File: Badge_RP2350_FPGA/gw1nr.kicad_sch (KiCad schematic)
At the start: 18 parts, among them U2 GW1N-LV9QN88C6_I5_, U6 W25Q32JVSS

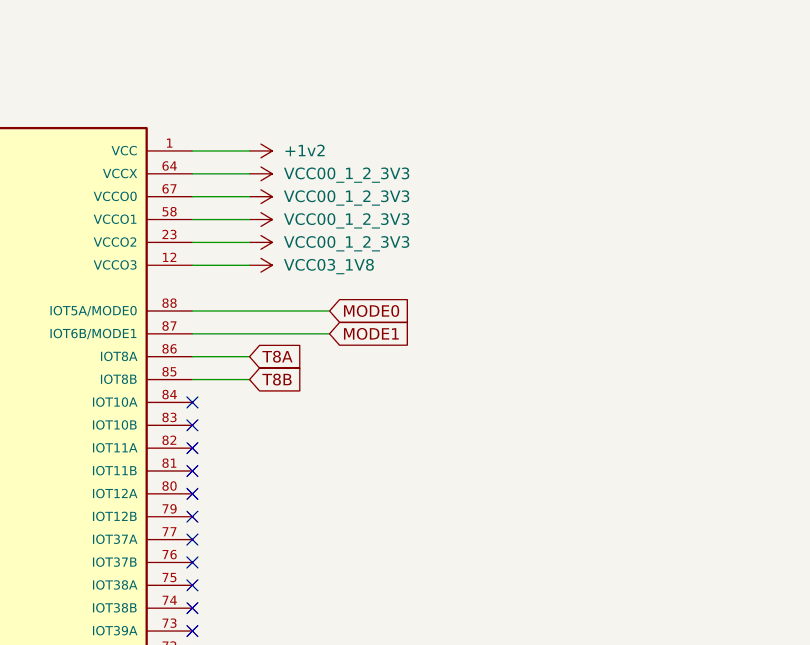
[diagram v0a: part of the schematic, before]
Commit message: put pull up to mode1, pull down to mode0
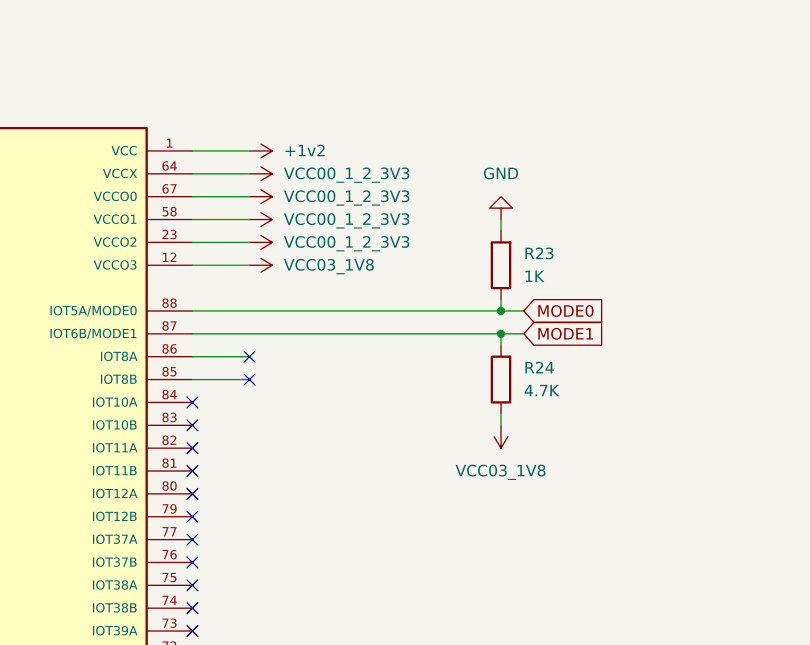
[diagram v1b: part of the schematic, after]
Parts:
- added R23: 1K, Resistor_SMD:R_0402_1005Metric, symbol Device:R
- added R24: 4.7K, Resistor_SMD:R_0402_1005Metric, symbol Device:R
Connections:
- net GND: now also R23.2
- net MODE0: now also R23.1
- net MODE1: now also R24.2
- net VCC03_1V8: now also R24.1
- net T8A: no longer names the net of U2.86 (IOT8A)
- net T8B: no longer names the net of U2.85 (IOT8B)
- no-connect marks 45 -> 47
